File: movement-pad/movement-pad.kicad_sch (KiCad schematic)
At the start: 32 parts

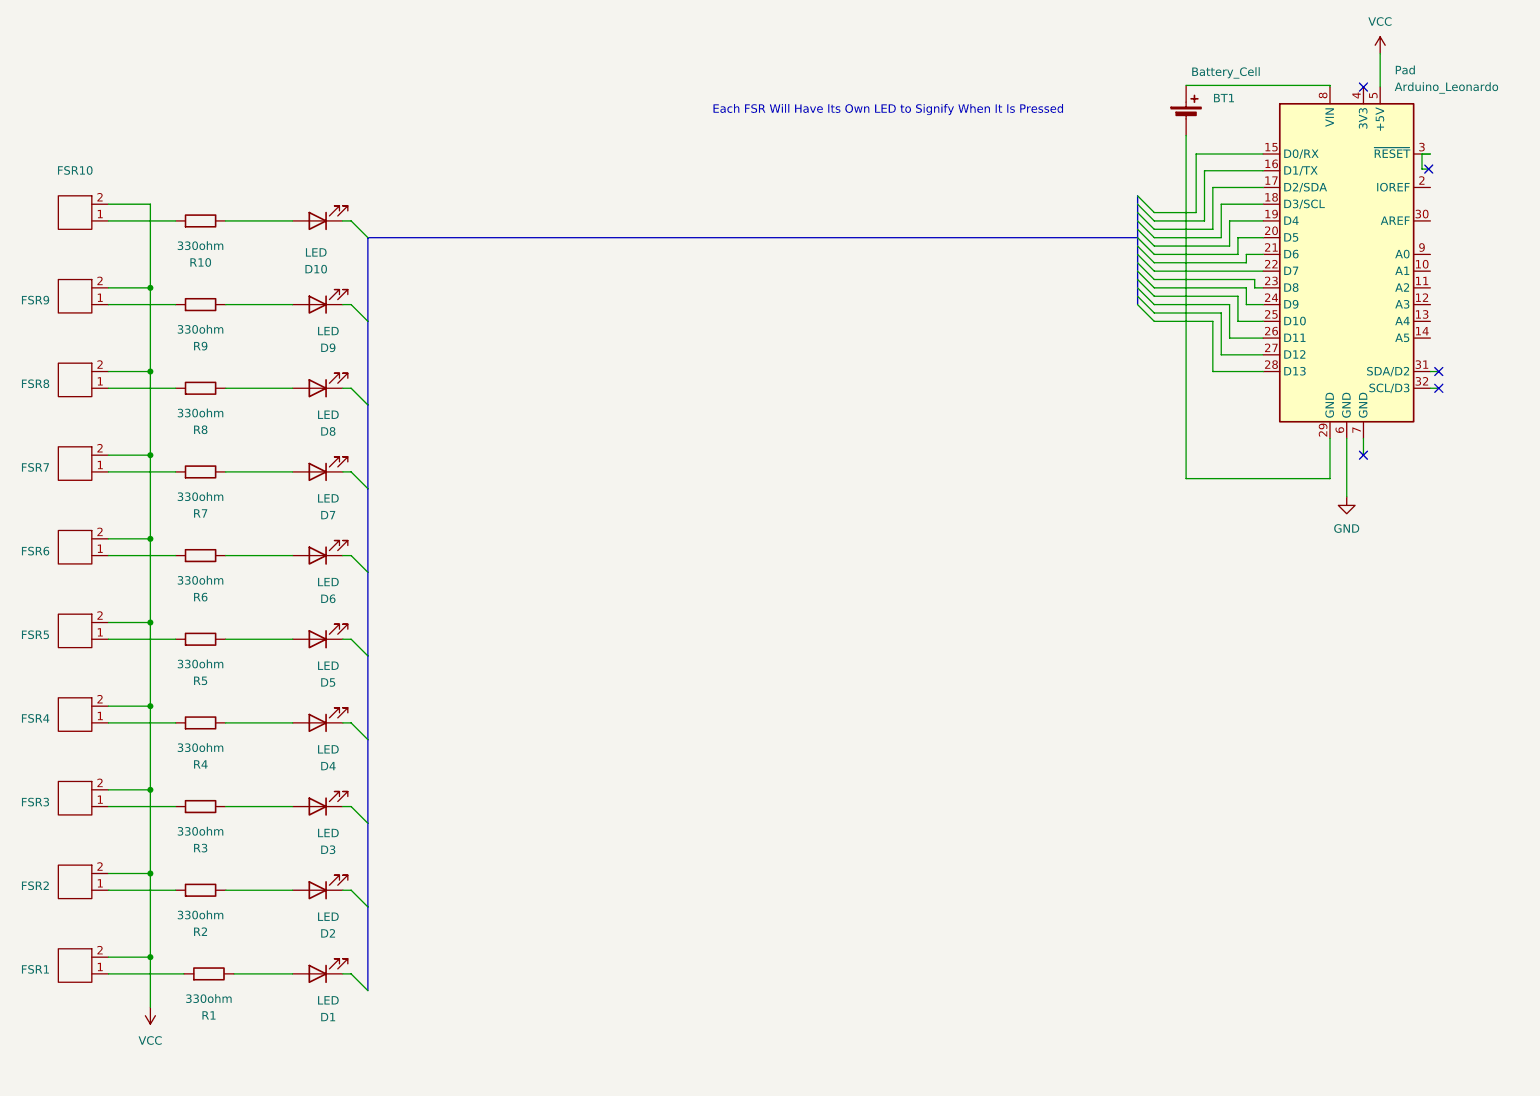
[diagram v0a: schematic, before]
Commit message: updated schematic
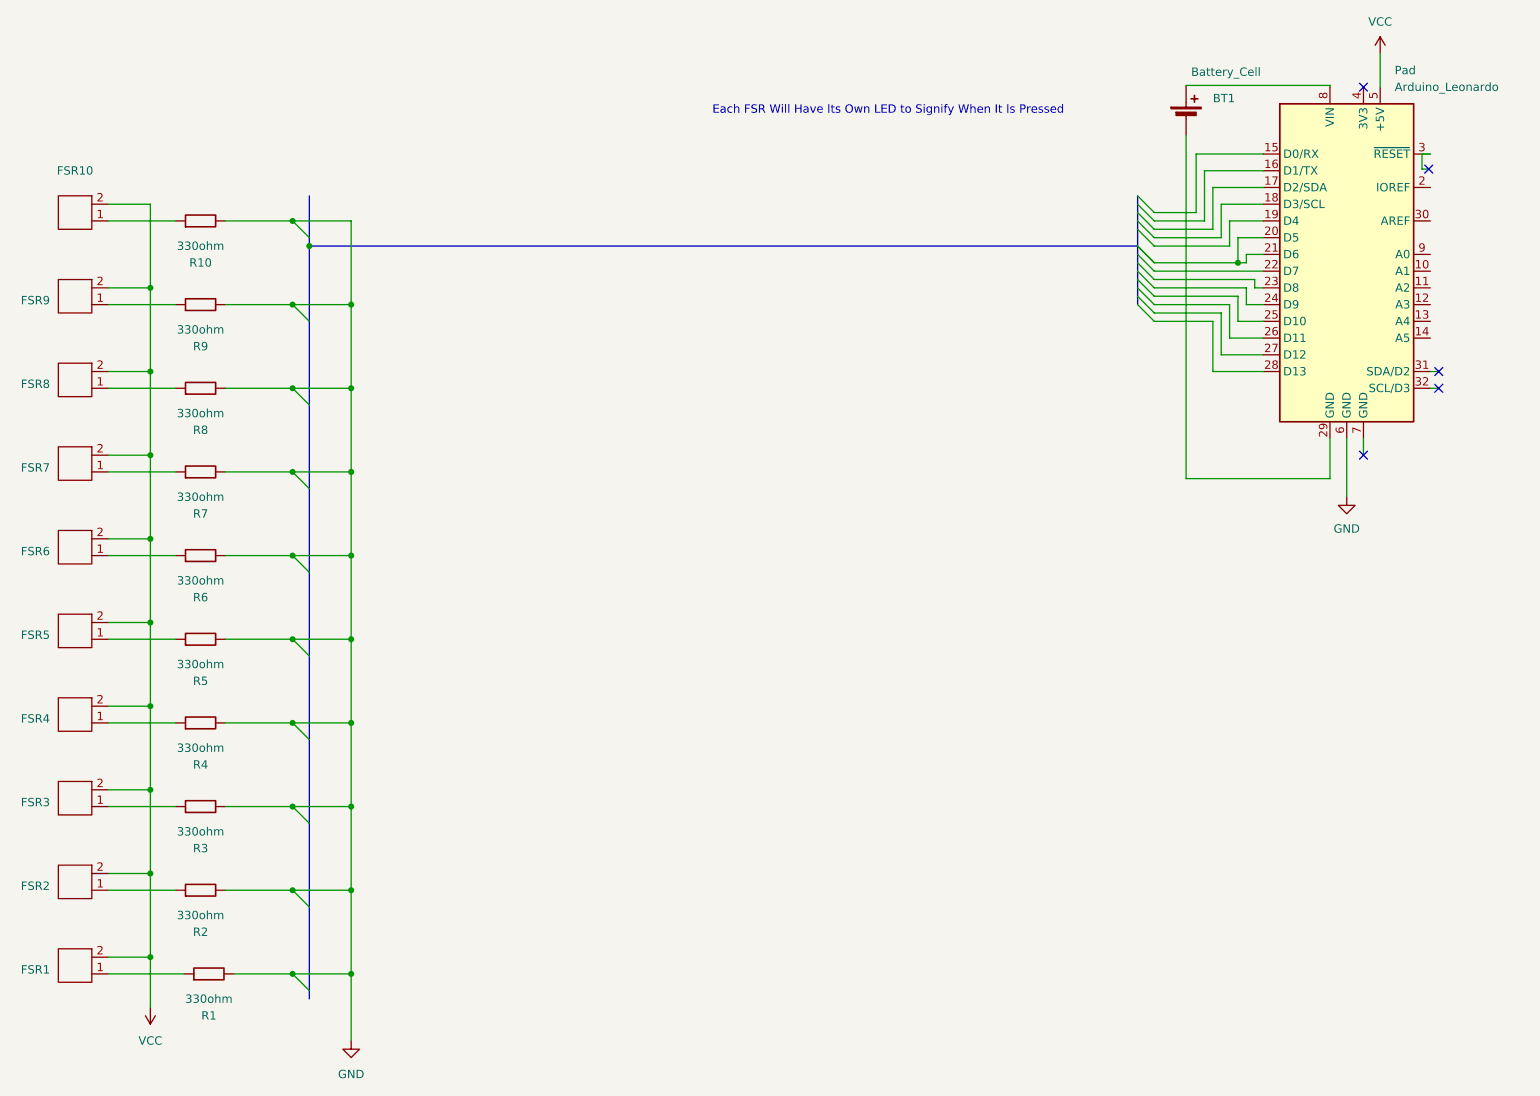
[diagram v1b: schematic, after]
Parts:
- removed D1, D10, D2, D3, D4, D5, D6, D7, D8, D9: LED, symbol Device:LED
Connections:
- net GND: now also R1.2, R10.2, R2.2, R3.2, R4.2, R5.2, R6.2, R7.2, R8.2, R9.2
- net at Pad.20 (D5): now also Pad.21 (D6)
